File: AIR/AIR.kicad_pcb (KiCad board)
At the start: 2 copper layers, 70.5 x 63 mm, 24 parts, among them P1 Conn_01x04_Pin, SW1 SW_Push_Dual, SW2 SW_Push_Dual, U1 ESP32-WROOM-32D, U2 TLV61046ADBVR, U3 INA219BIDR, U4 BME680

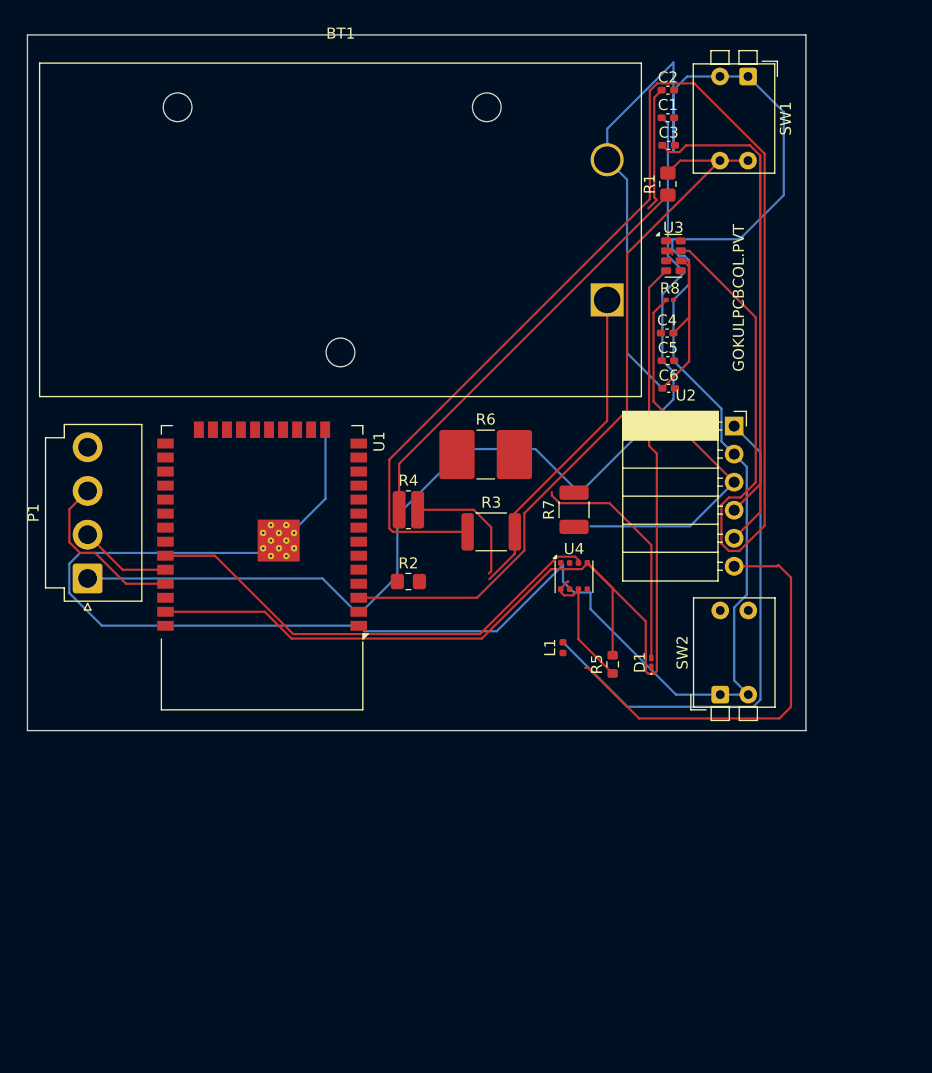
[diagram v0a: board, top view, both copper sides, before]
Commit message: error free version
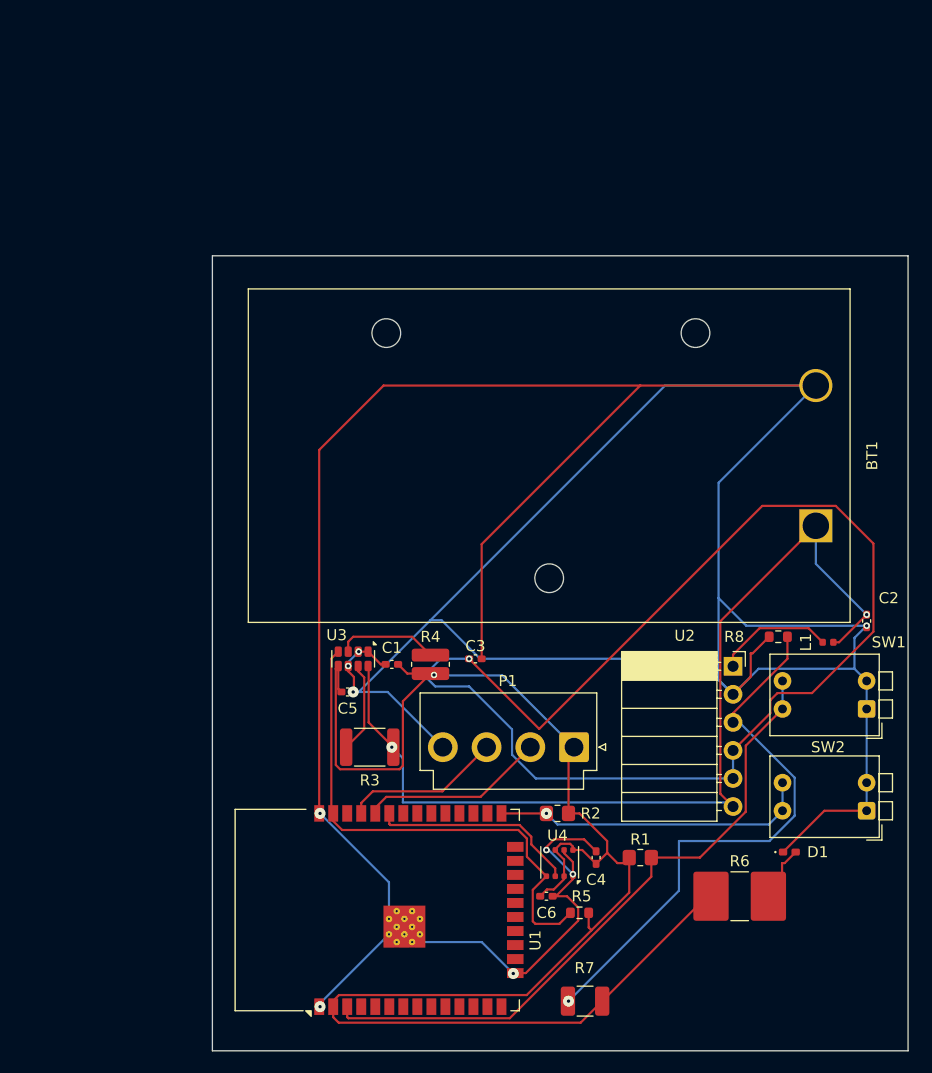
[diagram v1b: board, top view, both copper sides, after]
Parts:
- D1: footprint LED_SMD:LED_0201_0603Metric_Pad0.64x0.40mm_HandSolder -> LED_SMD:LED_0402_1005Metric_Pad0.77x0.64mm_HandSolder
- R8: footprint Resistor_SMD:R_0201_0603Metric -> Resistor_SMD:R_0603_1608Metric
- moved R1 61.1 mm to (138.5, 103.5), turned to 0 degrees
- moved SW1 58.3 mm to (159.0, 90.0), turned to 180 degrees
- moved C1 55.5 mm to (116.0, 86.0), turned to 180 degrees
- moved C2 51.3 mm to (159.0, 82.1), turned to -90 degrees
- moved C3 49.7 mm to (123.6, 85.5)
- moved C4 47.9 mm to (134.5, 103.5), turned to 90 degrees
- moved C6 47.3 mm to (130.0, 107.0), turned to 180 degrees
- moved P1 46.6 mm to (132.5, 93.5), turned to 180 degrees
- moved U3 46.6 mm to (112.5, 85.5), turned to -90 degrees
- moved R6 46.1 mm to (147.5, 107.0)
- moved R7 44.5 mm to (133.5, 116.5), turned to 0 degrees
- moved C5 41.7 mm to (112.0, 88.5)
- moved U1 36.5 mm to (117.7, 108.2), turned to 90 degrees
- moved R8 32.0 mm to (151.0, 83.5), turned to 180 degrees
- moved BT1 27.8 mm to (154.4, 73.5)
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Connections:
- P1 pad 4: <NO NET> -> GND
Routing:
- net /VIN: track 140.4 -> 8.26 mm
- net GND: track 253.2 -> 379.5 mm, vias 0 -> 9
- net /SCL: track 101.8 -> 46.8 mm
- net /3V3: track 78.5 -> 115.1 mm, vias 0 -> 1
- net Net-(U2-SW): track 46.3 -> 10.7 mm
- net /IO0: track 0.00 -> 28.9 mm, vias 0 -> 1
- net /SDA: track 43.6 -> 18.8 mm
- net /FB: track 34.7 -> 51.0 mm, vias 0 -> 1
- net Net-(D1-A): track 21.4 -> 5.16 mm
- net /RXD: track 8.36 -> 16.8 mm
- net /EN: track 67.1 -> 59.1 mm
- net /VCC: track 79.5 -> 87.3 mm, vias 0 -> 2
- net Net-(U3-SDA): track 11.6 -> 9.23 mm
- net +3V3: track 147.7 -> 149.4 mm, vias 0 -> 1
- net /TXD: track 15.6 -> 14.4 mm
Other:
- board size 70.5 x 63 mm -> 63 x 72 mm
- board text removed: "GOKULPCBCOL.PVT"
